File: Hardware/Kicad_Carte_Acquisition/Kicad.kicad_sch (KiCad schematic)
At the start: 42 parts, among them P1 DA15_Receptacle_MountingHoles, U1 TMP-15-215, U2 LM2937xS

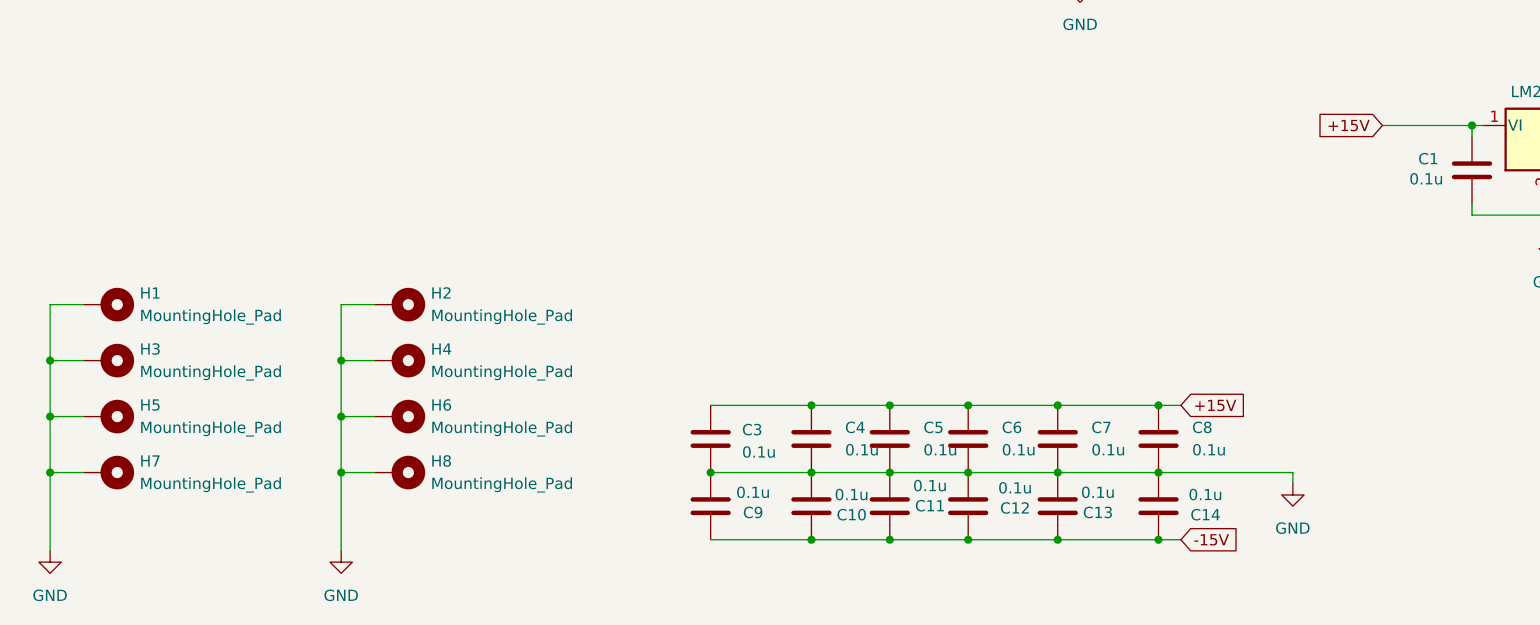
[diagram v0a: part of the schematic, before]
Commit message: modif
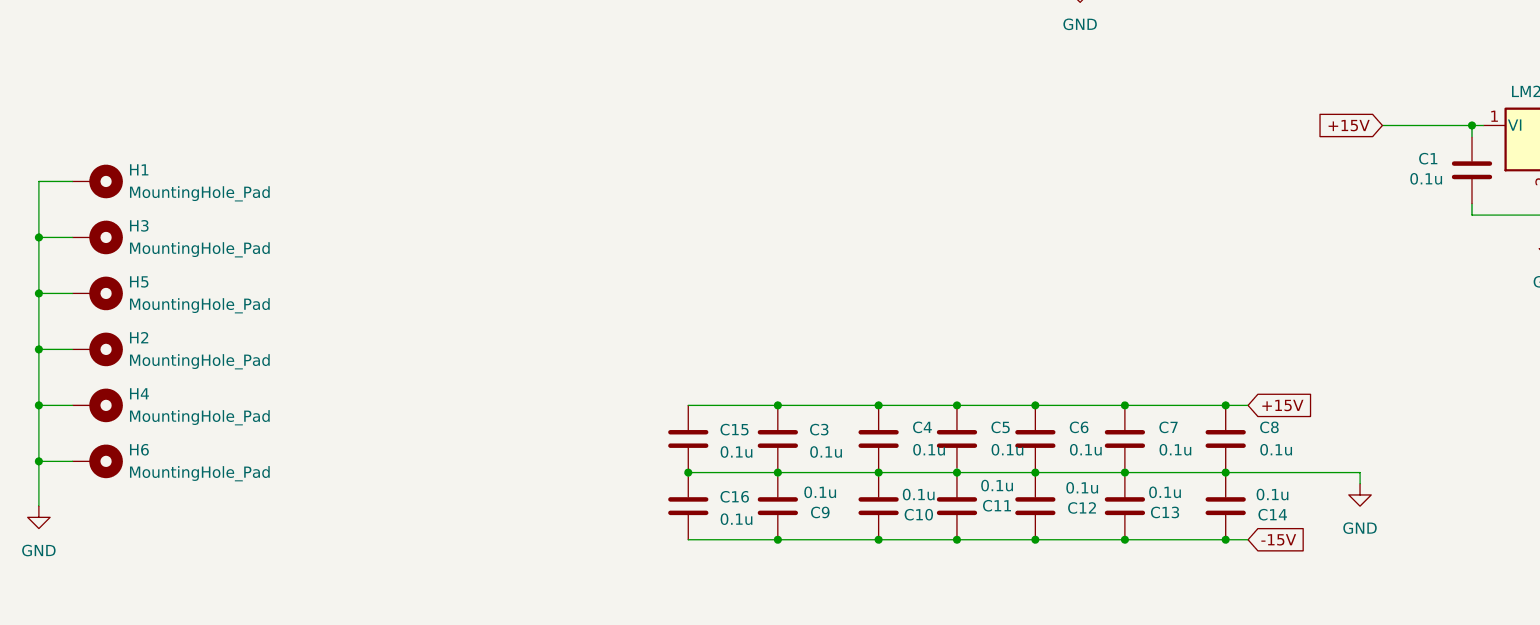
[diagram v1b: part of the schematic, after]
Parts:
- removed H6, H7: MountingHole_Pad, MountingHole:MountingHole_3.2mm_M3_Pad, symbol Mechanical:MountingHole_Pad
- added C15, C16: 0.1u, Capacitor_SMD:C_0603_1608Metric_Pad1.08x0.95mm_HandSolder, symbol Device:C
- renumbered H8 to H6
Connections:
- net +15V: now also C15.1
- net -15V: now also C16.2
- net GND: now also C15.2, C16.1
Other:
- moved on the sheet: C10, C11, C12, C13, C14, C3, C4, C5, C6, C7, C8, C9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

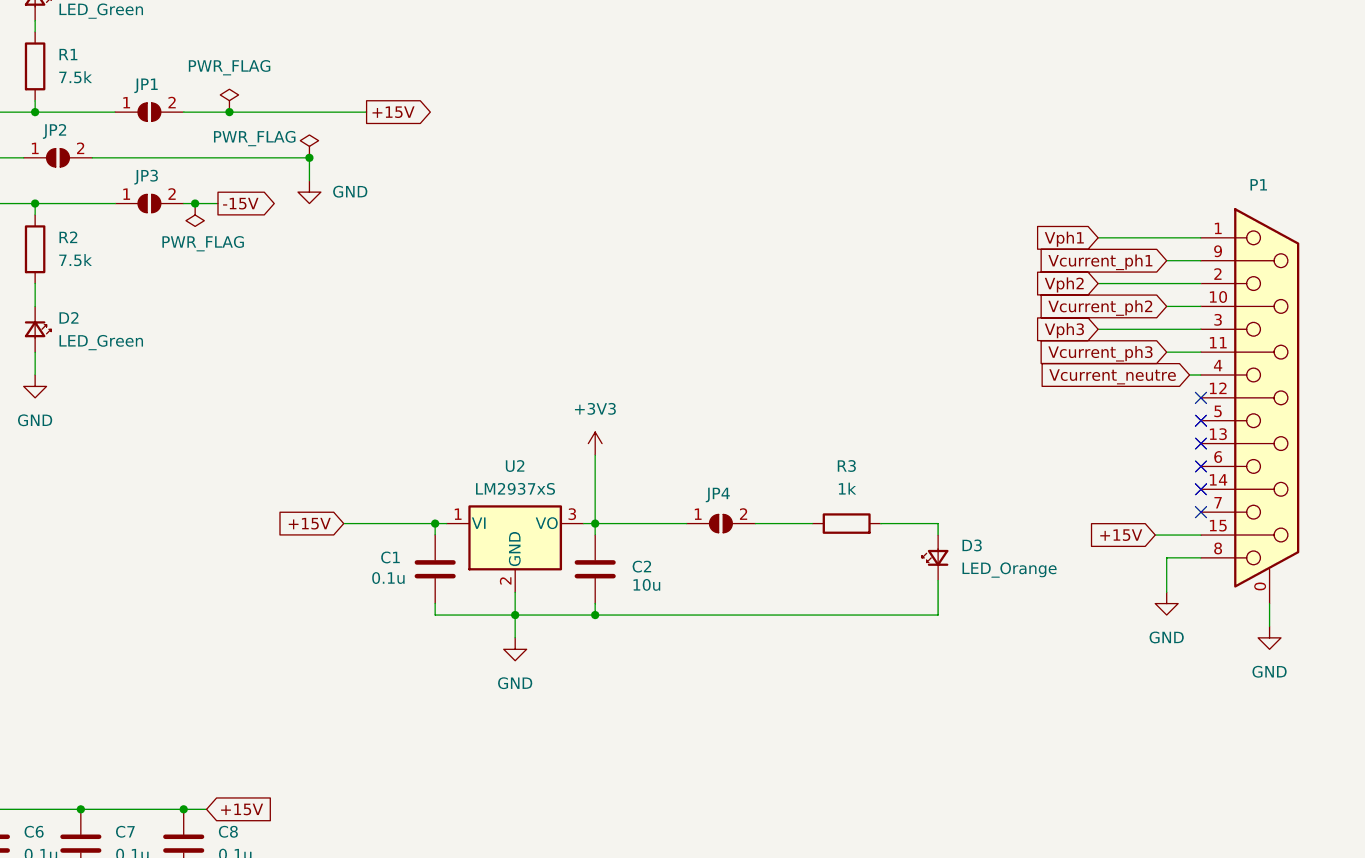
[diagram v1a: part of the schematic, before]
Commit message: modif
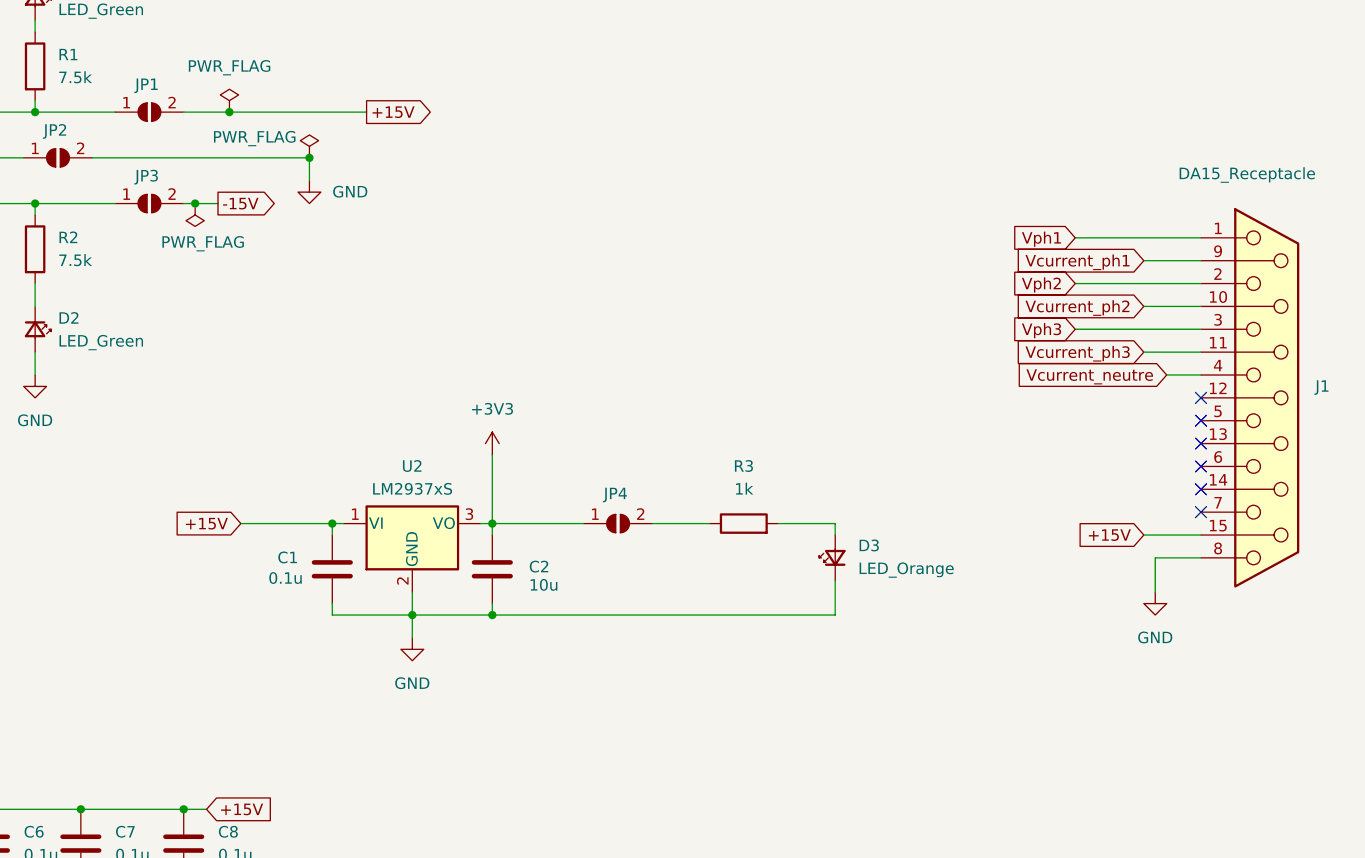
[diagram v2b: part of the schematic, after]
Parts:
- removed P1: DA15_Receptacle_MountingHoles, Library.pretty_Dsub_15_Female:Dsub_15_Female_E, symbol Connector:DA15_Receptacle_MountingHoles
- added J1: DA15_Receptacle, Library.pretty_SUBD_F:618015231321, symbol Connector:DA15_Receptacle
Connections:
- net +15V: now also J1.15 (P15)
- net GND: now also J1.8
- net Vcurrent_neutre: now also J1.4
- net Vcurrent_ph1: now also J1.9 (P9)
- net Vcurrent_ph2: now also J1.10 (P10)
- net Vcurrent_ph3: now also J1.11 (P111)
- net Vph1: now also J1.1
- net Vph2: now also J1.2
- net Vph3: now also J1.3
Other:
- moved on the sheet: C1, C2, D3, JP4, R3, U2
